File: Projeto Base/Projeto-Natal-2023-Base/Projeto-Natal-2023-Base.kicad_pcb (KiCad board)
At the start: 2 copper layers, 77.8 x 77.8 mm, 71 parts, among them J1 Conn_01x01_Pin, J2 Conn_01x01_Pin, J3 Conn_01x01_Pin, J4 Conn_01x01_Pin, J5 Conn_01x01_Pin, J6 Conn_01x01_Pin, J7 Conn_01x01_Pin, J8 Conn_01x01_Pin, Q1 BC817, Q2 BC817, Q3 BC817, Q4 BC817, Q5 MMBT3906, SW1 SW_Push, SW2 SW_Push, U1 CH32V003F4P6

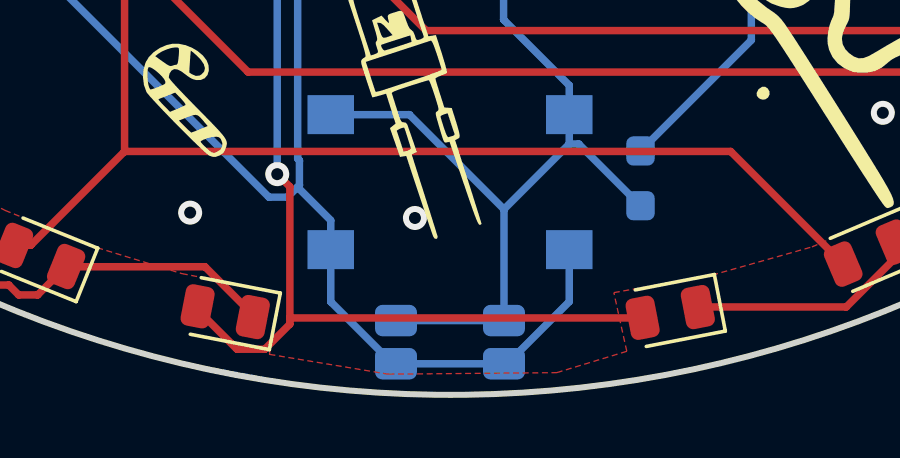
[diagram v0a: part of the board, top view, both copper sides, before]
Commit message: update files
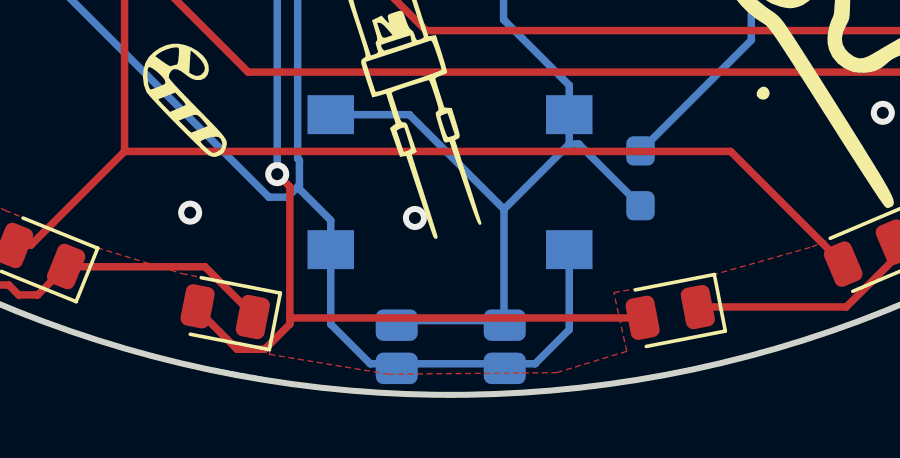
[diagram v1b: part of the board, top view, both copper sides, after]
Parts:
- D1, D10, D13, D18, D21, D24, D27, D30, D4, D7: value LED -> D-B080508B1-KS2
- D11, D14, D17, D2, D20, D23, D26, D29, D5, D8: value LED -> e17-21SURC/S530-A3/TR8
- D12, D15, D16, D19, D22, D25, D28, D3, D6, D9: value LED -> NCD0805G1
- SW1: value SW_Push -> EVQP7A
- moved SW1 0.15 mm to (94.0, 136.3)
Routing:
- net GND: track 211.0 -> 212.0 mm
